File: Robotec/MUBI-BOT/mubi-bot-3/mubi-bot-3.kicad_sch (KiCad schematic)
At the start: 10 parts, among them IC1 L293E, X1 AK500/10-H, X2 AK500/10-H

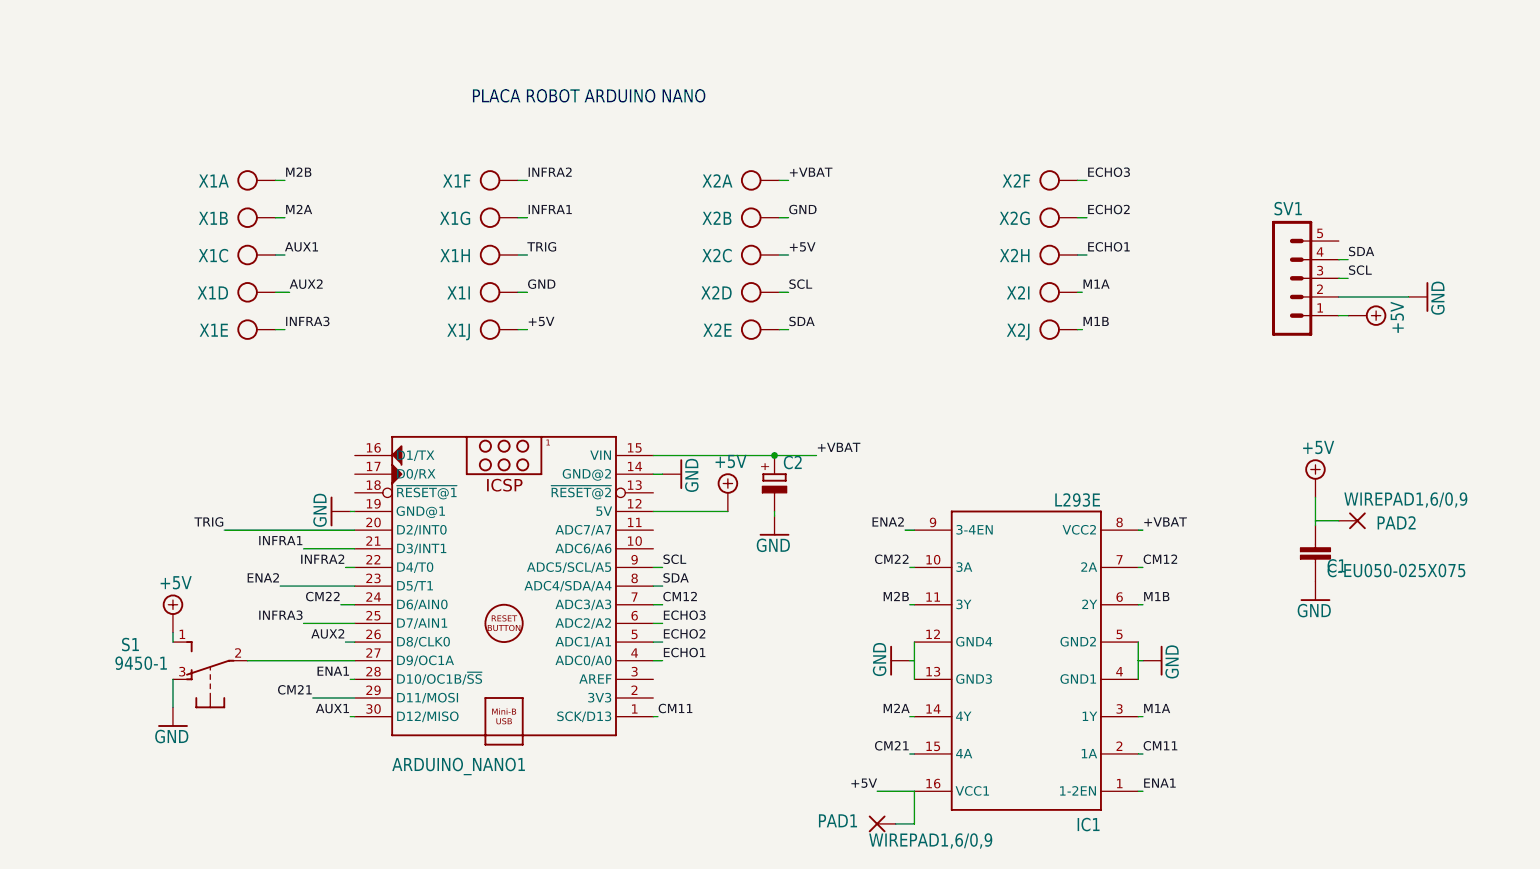
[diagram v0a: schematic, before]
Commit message: update sch pcb kicad v9
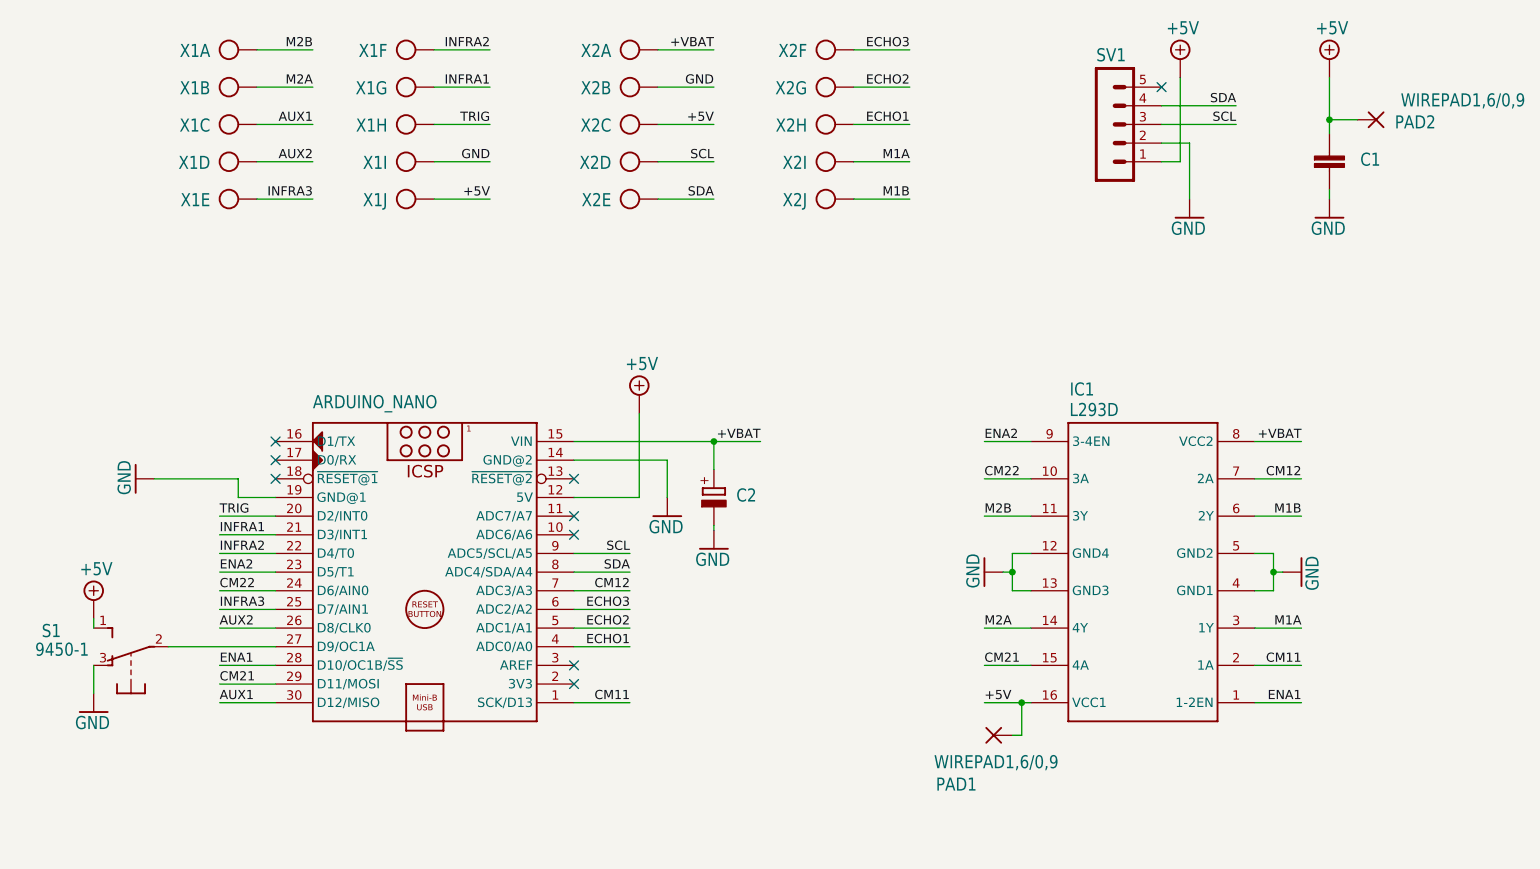
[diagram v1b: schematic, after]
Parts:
- IC1: value L293E -> L293D
- renumbered ARDUINO_NANO1 to ARDUINO_NANO
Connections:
- no-connect marks 0 -> 9
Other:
- note removed: "PLACA ROBOT ARDUINO NANO"
- company: (none) -> E.E.S.T. N.°5 "AMANCIO WILLIAMS"
- title: (none) -> MUBI-BOT NANO v4
- moved on the sheet: ARDUINO_NANO, C1, C2, IC1, PAD1, PAD2, S1, SV1, X1A, X1B, X1C, X1D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
